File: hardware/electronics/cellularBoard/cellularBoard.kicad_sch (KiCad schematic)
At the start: 15 parts, among them J1 Standoff, J2 M.2_E_Key_PCB_Edge, U1 LM51571-Q1

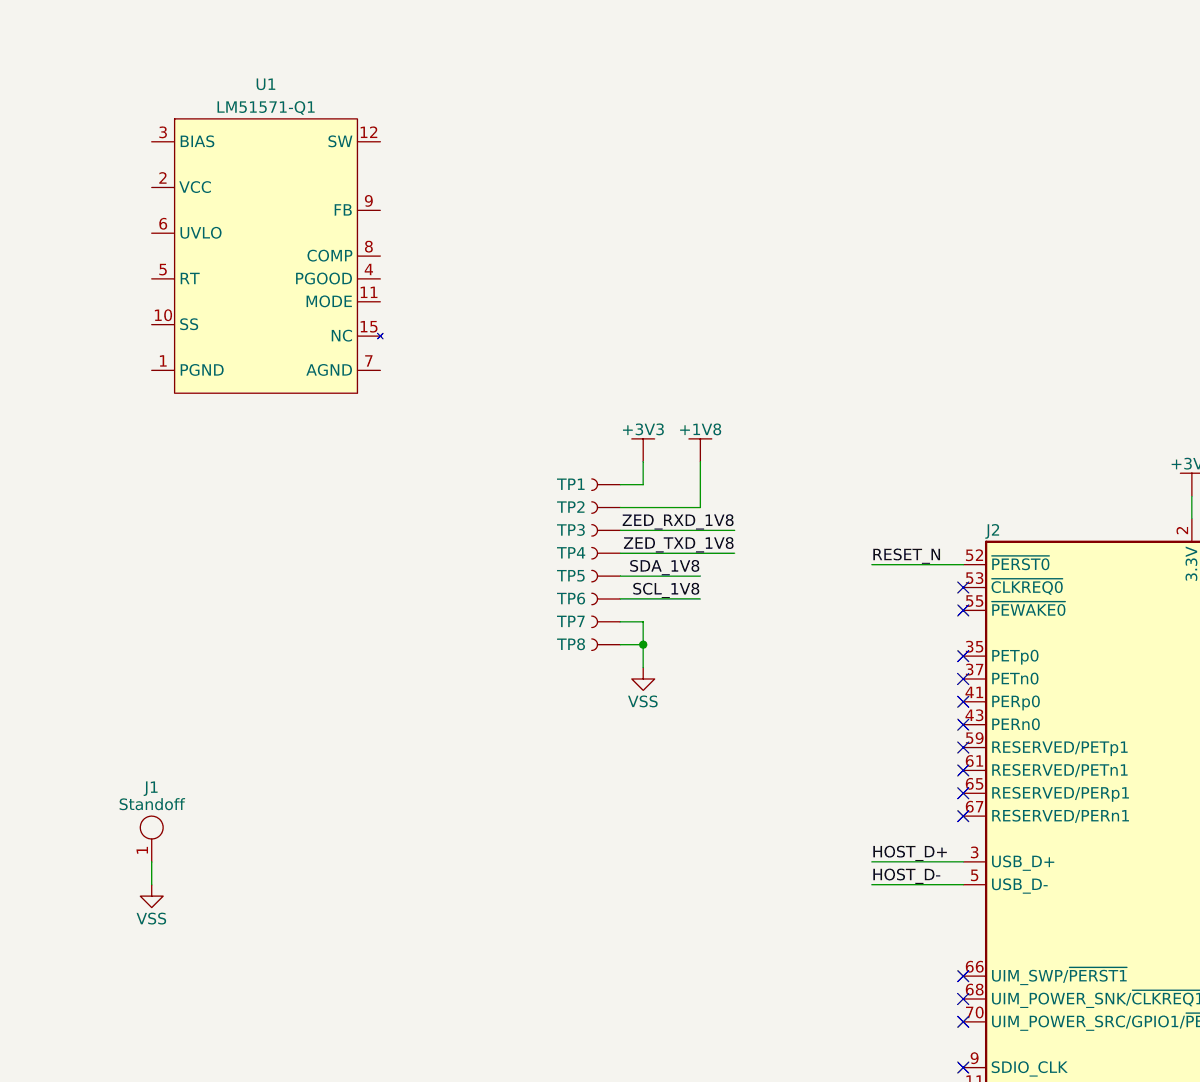
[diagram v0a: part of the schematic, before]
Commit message: started on schematics
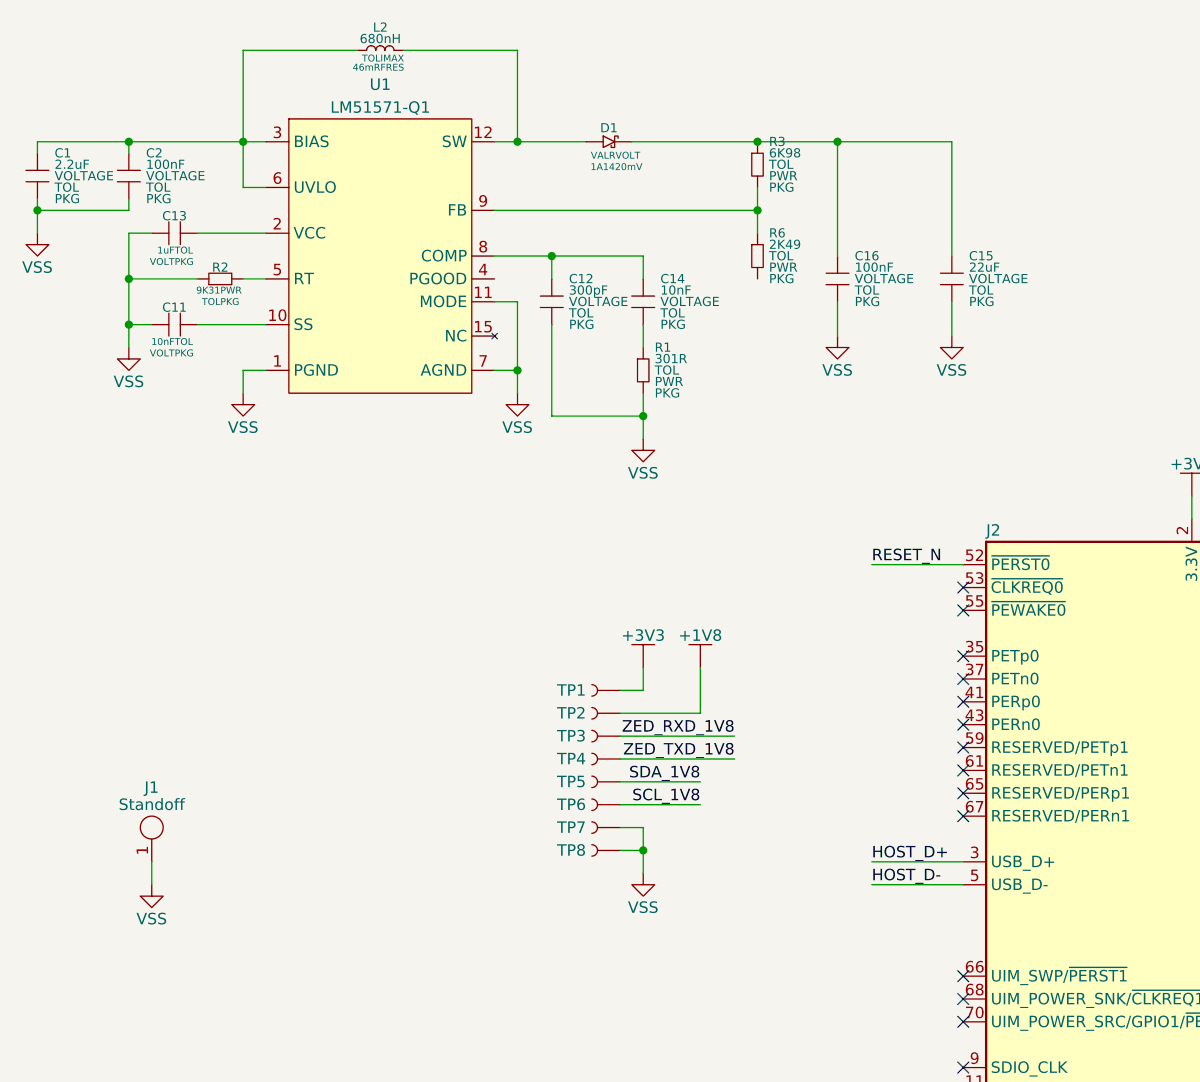
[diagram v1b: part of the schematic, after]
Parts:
- added C1: 2.2uF, symbol lib_sch:C
- added C11: 10nF, symbol lib_sch:C_horizontal
- added C12: 300pF, symbol lib_sch:C
- added C13: 1uF, symbol lib_sch:C_horizontal
- added C14: 10nF, symbol lib_sch:C
- added C15: 22uF, symbol lib_sch:C
- added C16, C2: 100nF, symbol lib_sch:C
- added D1: VAL, symbol DS-Diodes:D_Schottky_horizontal
- added L2: 680nH, symbol DS-Passives:L_horizontal
- added R1: 301R, symbol lib_sch:R
- added R2: 9K31, symbol lib_sch:R_horizontal
- added R3: 6K98, symbol lib_sch:R
- added R6: 2K49, symbol lib_sch:R
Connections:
- net VSS: now also U1.1 (PGND), U1.11 (MODE), U1.16 (PGND), U1.17 (AGND), U1.7 (AGND), C1.2, C11.1, C12.2, C13.1, C15.2, C16.2, C2.2, R1.2, R2.1
- net at U1.10 (SS): now also C11.2
- net at U1.12 (SW), U1.13 (SW), U1.14 (SW): now also D1.1, L2.2
- net at U1.2 (VCC): now also C13.2
- net at U1.3 (BIAS): now also U1.6 (UVLO), C1.1, C2.1, L2.1
- net at U1.5 (RT): now also R2.2
- net at U1.8 (COMP): now also C12.1, C14.1
- net at U1.9 (FB): now also R3.2, R6.1
- new net: C14.2, R1.1
- new net: C15.1, C16.1, D1.2, R3.1
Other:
- moved on the sheet: TP1, TP2, TP3, TP4, TP5, TP6, TP7, TP8, U1
